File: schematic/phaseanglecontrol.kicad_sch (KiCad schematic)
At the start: 50 parts, among them J1 L_supply, J2 N_supply, J3 N_motor, J4 L_motor, K1 shutoff, U1 ATtiny26-16P, Y1 16 MHz

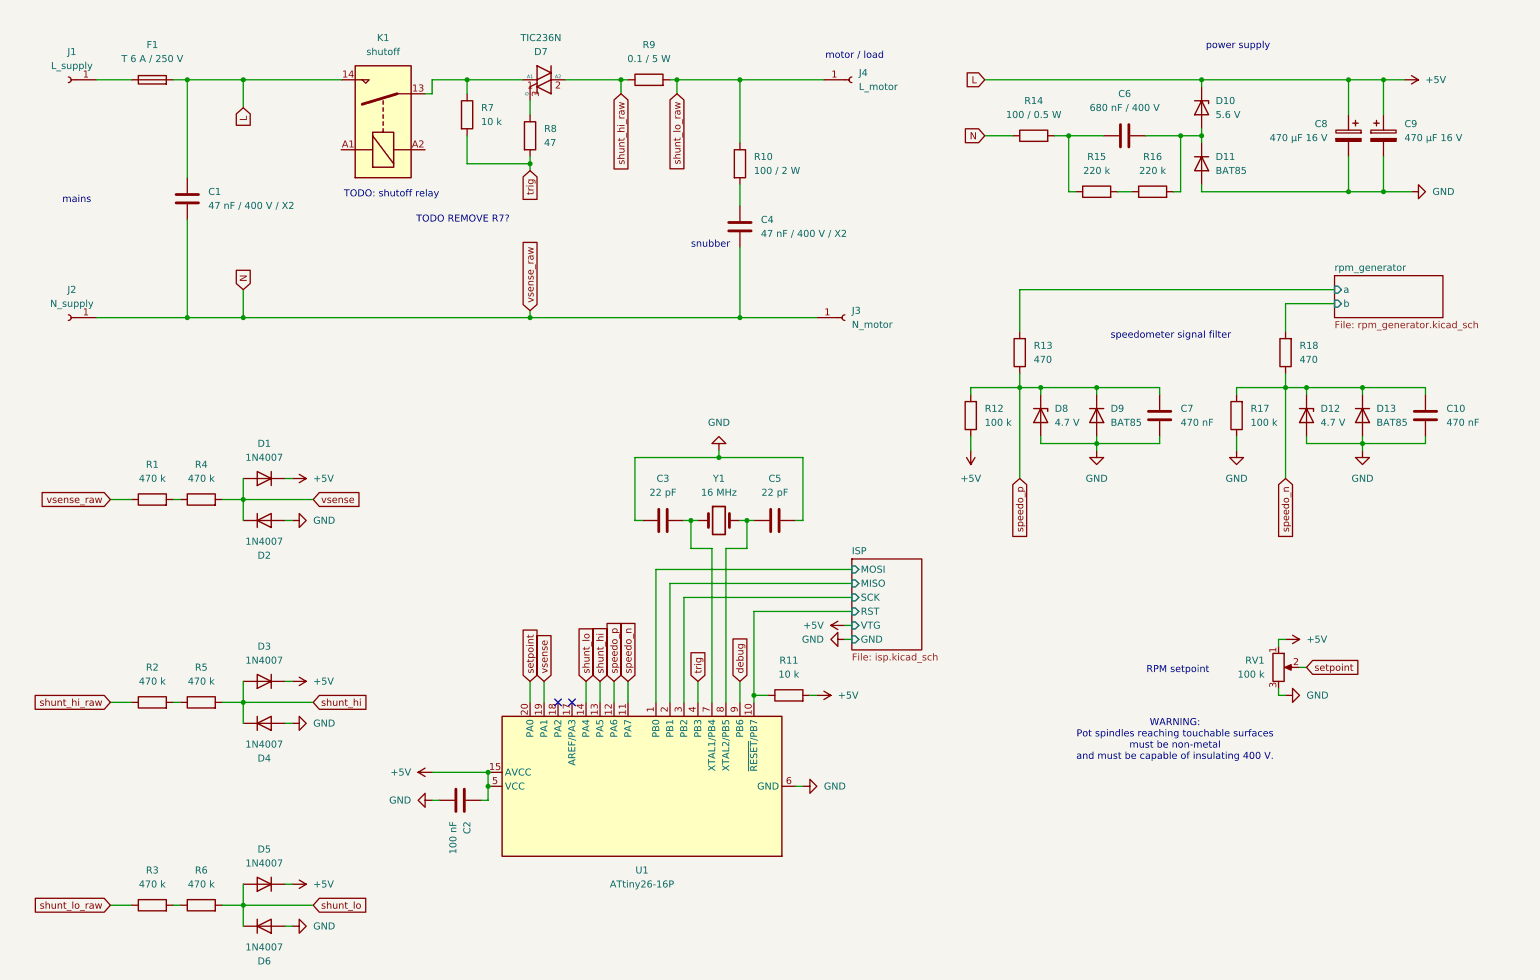
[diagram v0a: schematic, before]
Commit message: Update schematics
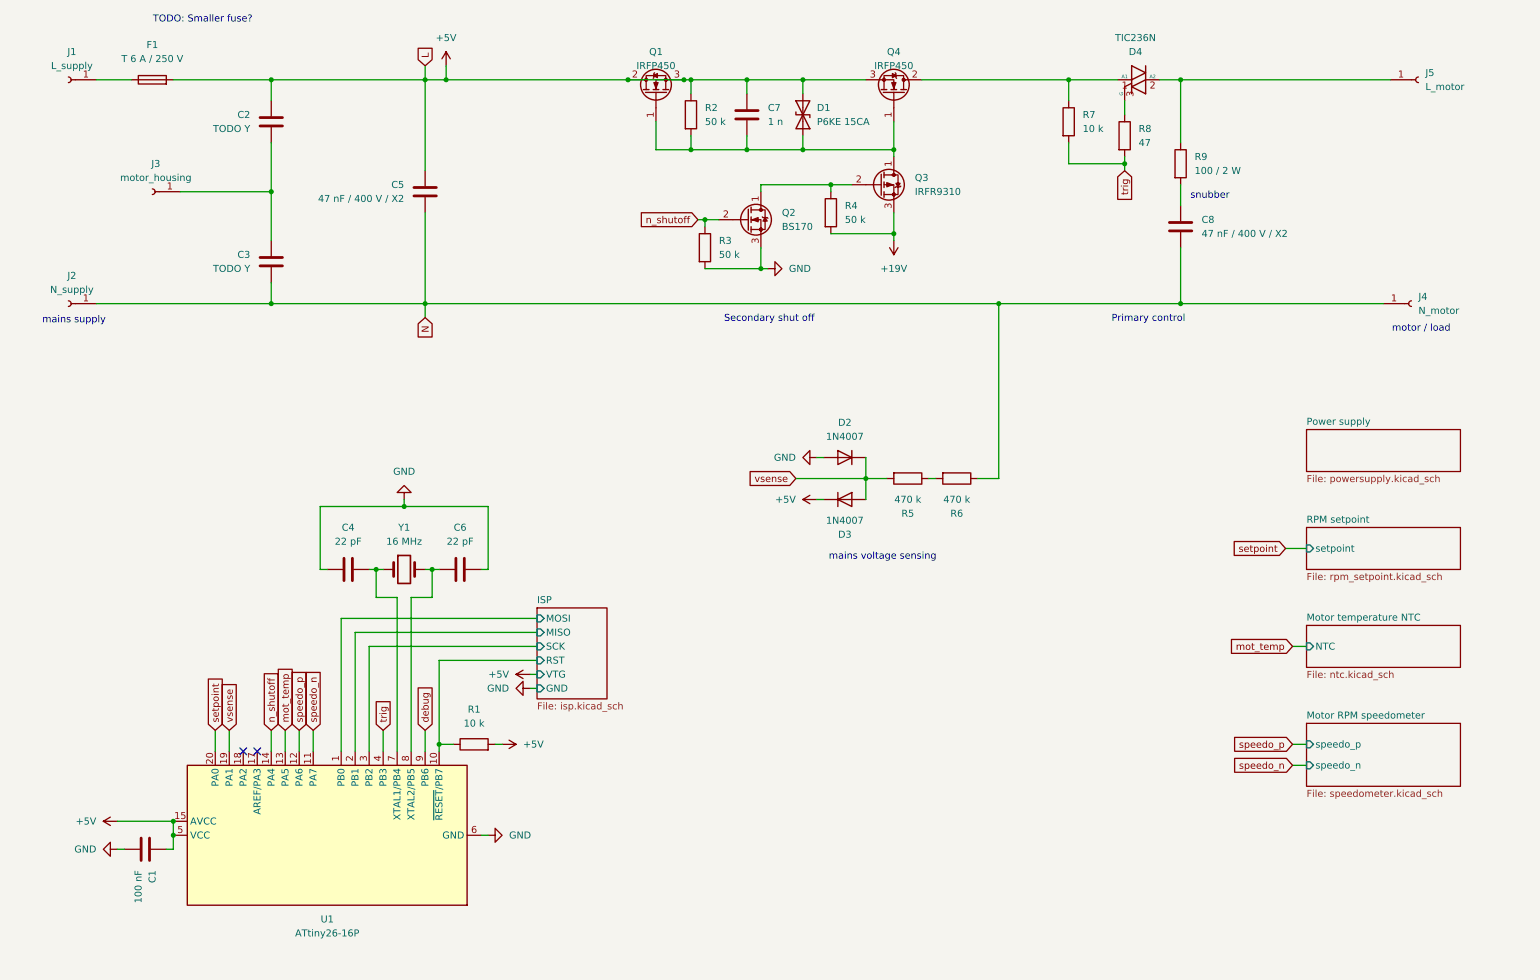
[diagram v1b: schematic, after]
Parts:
- removed C10: 470 nF, symbol Device:C
- removed C6: 680 nF / 400 V, symbol Device:C
- removed C8, C9: 470 µF 16 V, symbol Device:C_Polarized
- removed D10: 5.6 V, symbol Device:D_Zener
- removed D11, D13, D9: BAT85, symbol Device:D
- removed D12, D8: 4.7 V, symbol Device:D_Zener
- removed D3, D4, D5, D6: 1N4007, Diode_THT:D_DO-41_SOD81_P10.16mm_Horizontal, symbol Diode:1N4007
- removed K1: shutoff, symbol Relay:Relay_SPST-NO
- removed R12, R17: 100 k, symbol Device:R
- removed R13, R18: 470, symbol Device:R
- removed R14: 100 / 0.5 W, symbol Device:R
- removed R15, R16: 220 k, symbol Device:R
- removed R5, R6: 470 k, symbol Device:R
- removed R9: 0.1 / 5 W, symbol Device:R
- removed RV1: 100 k, symbol Device:R_Potentiometer
- added C2, C3: TODO Y, symbol Device:C
- added D1: P6KE 15CA, Diode_THT:D_DO-201AE_P15.24mm_Horizontal, symbol Diode:1N62xxCA
- added J3: motor_housing, symbol Connector:Conn_01x01_Socket
- added Q1, Q4: IRFP450, Package_TO_SOT_THT:TO-247-3_Vertical, symbol Transistor_FET:IRFP4468PbF
- added Q2: BS170, Package_TO_SOT_THT:TO-92_Inline, symbol Transistor_FET:BS170
- added Q3: IRFR9310, Package_TO_SOT_THT:TO-92_Inline, symbol Transistor_FET:BS250
- added R4: 50 k, symbol Device:R
- C7: value 470 nF -> 1 n
- R2, R3: value 470 k -> 50 k
- renumbered C2 to C1, C3 to C4, C1 to C5, C5 to C6, C4 to C8, D1 to D3, D7 to D4, J3 to J4, J4 to J5, R11 to R1, R4 to R5, R1 to R6, R10 to R9
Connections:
- net +5V: now also C7.1, R2.1, C2.2, D1.2 (A2), Q1.2 (D), Q1.3 (S), Q4.3 (S)
- net GND: now also R3.2, Q2.3 (S); no longer C7.2
- net N: now also C3.1
- net speedo_p: no longer C7.1
- net at D4.1 (A1), R7.1: now also Q4.2 (D)
- net at R2.2: now also C7.2, D1.1 (A1), Q1.1 (G), Q3.1 (D), Q4.1 (G)
- net shunt_hi renamed mot_temp
- net shunt_hi_raw: no longer names the net of D4.2 (A2)
- net shunt_hi_raw: now also J5.1 (Pin_1), R9.1; no longer R2.1
- net shunt_lo renamed n_shutoff
- net n_shutoff: now also R3.1, Q2.2 (G)
- removed net shunt_lo_raw: J5.1 (Pin_1), R3.1, R9.1
- new net: Q2.1 (D), Q3.2 (G), R4.1
- new net: C2.1, C3.2, J3.1 (Pin_1)
- new net +19V: Q3.3 (S), R4.2
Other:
- removed sheet rpm_generator
- added sheet Motor RPM speedometer (speedometer.kicad_sch)
- added sheet Motor temperature NTC (ntc.kicad_sch)
- added sheet Power supply (powersupply.kicad_sch)
- added sheet RPM setpoint (rpm_setpoint.kicad_sch)
- note added: "Primary control"
- note added: "Secondary shut off"
- note added: "TODO: Smaller fuse?"
- note added: "mains supply"
- note added: "mains voltage sensing"
- note removed: "RPM setpoint"
- note removed: "TODO REMOVE R7?"
- note removed: "TODO: shutoff relay"
- note removed: "WARNING: Pot spindles reaching touchable surfaces must be non-metal and must be capable of insulating 400 V."
- note removed: "mains"
- note removed: "power supply"
- note removed: "speedometer signal filter"
- moved on the sheet: C1, C4, C5, C6, C8, D2, D3, D4, J2, J4, J5, R1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

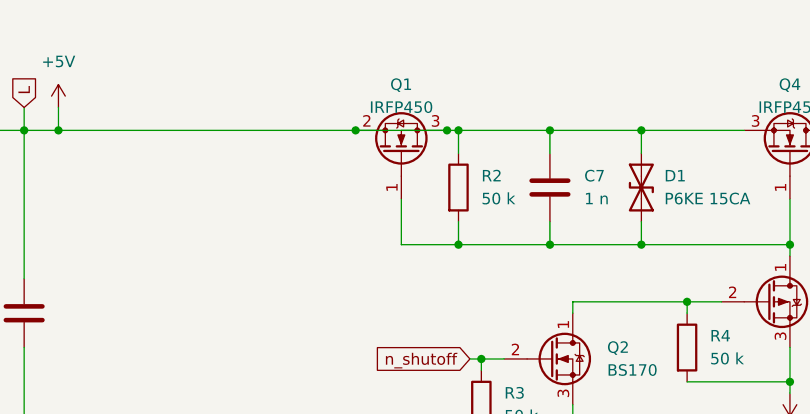
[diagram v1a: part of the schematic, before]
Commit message: Update schematic
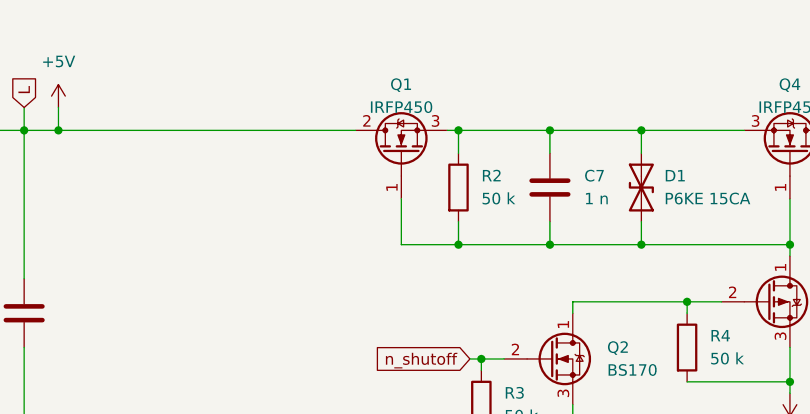
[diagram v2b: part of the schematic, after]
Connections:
- net +5V: no longer C7.1, D1.2 (A2), Q1.3 (S), Q4.3 (S), R2.1
- new net: C7.1, D1.2 (A2), Q1.3 (S), Q4.3 (S), R2.1
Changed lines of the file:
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@@
 	)
 	(junction
-		(at 135.89 27.94)
+		(at 137.16 27.94)
 		(diameter 0)
 		(color 0 0 0 0)
@@
 	)
 	(junction
-		(at 137.16 27.94)
-		(diameter 0)
-		(color 0 0 0 0)
-	)
-	(junction
 		(at 173.99 40.64)
 		(diameter 0)
@@
 	)
 	(junction
-		(at 125.73 27.94)
+		(at 92.71 27.94)
 		(diameter 0)
 		(color 0 0 0 0)
@@
 	(junction
 		(at 226.06 27.94)
-		(diameter 0)
-		(color 0 0 0 0)
-	)
-	(junction
-		(at 92.71 27.94)
 		(diameter 0)
 		(color 0 0 0 0)
@@
 	(wire
 		(pts
+			(xy 162.56 55.88) (xy 173.99 55.88)
+		)
+		(stroke
+			(width 0)
+			(type default)
+		)
+	)
+	(wire
+		(pts
+			(xy 222.25 27.94) (xy 226.06 27.94)
+		)
+		(stroke
+			(width 0)
+			(type default)
+		)
+	)
+	(wire
+		(pts
+			(xy 43.18 167.64) (xy 41.91 167.64)
+		)
+		(stroke
+			(width 0)
+			(type default)
+		)
+	)
+	(wire
+		(pts
+			(xy 149.86 62.23) (xy 151.13 62.23)
+		)
+		(stroke
+			(width 0)
+			(type default)
+		)
+	)
+	(wire
+		(pts
+			(xy 193.04 100.33) (xy 189.23 100.33)
+		)
+		(stroke
+			(width 0)
+			(type default)
+		)
+	)
+	(wire
+		(pts
+			(xy 130.81 40.64) (xy 137.16 40.64)
+		)
+		(stroke
+			(width 0)
+			(type default)
+		)
+	)
+	(wire
+		(pts
+			(xy 33.02 167.64) (xy 34.29 167.64)
+		)
+		(stroke
+			(width 0)
+			(type default)
+		)
+	)
+	(wire
+		(pts
+			(xy 173.99 40.64) (xy 173.99 35.56)
+		)
+		(stroke
+			(width 0)
+			(type default)
+		)
+	)
+	(wire
+		(pts
+			(xy 168.91 104.14) (xy 168.91 100.33)
+		)
+		(stroke
+			(width 0)
+			(type default)
+		)
+	)
+	(wire
+		(pts
+			(xy 83.82 121.92) (xy 83.82 149.86)
+		)
+		(stroke
+			(width 0)
+			(type default)
+		)
+	)
+	(wire
+		(pts
+			(xy 60.96 27.94) (xy 60.96 31.75)
+		)
+		(stroke
+			(width 0)
+			(type default)
+		)
+	)
+	(wire
+		(pts
+			(xy 157.48 27.94) (xy 168.91 27.94)
+		)
+		(stroke
+			(width 0)
+			(type default)
+		)
+	)
+	(wire
+		(pts
+			(xy 172.72 100.33) (xy 168.91 100.33)
+		)
+		(stroke
+			(width 0)
+			(type default)
+		)
+	)
+	(wire
+		(pts
+			(xy 90.17 121.92) (xy 86.36 121.92)
+		)
+		(stroke
+			(width 0)
+			(type default)
+		)
+	)
+	(wire
+		(pts
+			(xy 168.91 100.33) (xy 156.21 100.33)
+		)
+		(stroke
+			(width 0)
+			(type default)
+		)
+	)
+	(wire
+		(pts
+			(xy 226.06 58.42) (xy 226.06 68.58)
+		)
+		(stroke
+			(width 0)
+			(type default)
+		)
+	)
+	(wire
+		(pts
+			(xy 68.58 146.05) (xy 68.58 149.86)
+		)
+		(stroke
+			(width 0)
+			(type default)
+		)
+	)
+	(wire
+		(pts
+			(xy 43.18 27.94) (xy 60.96 27.94)
+		)
+		(stroke
+			(width 0)
+			(type default)
+		)
+	)
+	(wire
+		(pts
+			(xy 43.18 162.56) (xy 43.18 165.1)
+		)
+		(stroke
+			(width 0)
+			(type default)
+		)
+	)
+	(wire
+		(pts
+			(xy 205.74 39.37) (xy 205.74 43.18)
+		)
+		(stroke
+			(width 0)
+			(type default)
+		)
+	)
+	(wire
+		(pts
+			(xy 60.96 27.94) (xy 88.9 27.94)
+		)
+		(stroke
+			(width 0)
+			(type default)
+		)
+	)
+	(wire
+		(pts
 			(xy 92.71 27.94) (xy 125.73 27.94)
 		)
@@
 	(wire
 		(pts
-			(xy 162.56 55.88) (xy 173.99 55.88)
-		)
-		(stroke
-			(width 0)
-			(type default)
-		)
-	)
-	(wire
-		(pts
-			(xy 222.25 27.94) (xy 226.06 27.94)
-		)
-		(stroke
-			(width 0)
-			(type default)
-		)
-	)
-	(wire
-		(pts
-			(xy 137.16 27.94) (xy 135.89 27.94)
-		)
-		(stroke
-			(width 0)
-			(type default)
-		)
-	)
-	(wire
-		(pts
-			(xy 43.18 167.64) (xy 41.91 167.64)
-		)
-		(stroke
-			(width 0)
-			(type default)
-		)
-	)
-	(wire
-		(pts
-			(xy 149.86 62.23) (xy 151.13 62.23)
-		)
-		(stroke
-			(width 0)
-			(type default)
-		)
-	)
-	(wire
-		(pts
-			(xy 193.04 100.33) (xy 189.23 100.33)
-		)
-		(stroke
-			(width 0)
-			(type default)
-		)
-	)
-	(wire
-		(pts
-			(xy 130.81 40.64) (xy 137.16 40.64)
-		)
-		(stroke
-			(width 0)
-			(type default)
-		)
-	)
-	(wire
-		(pts
-			(xy 33.02 167.64) (xy 34.29 167.64)
-		)
-		(stroke
-			(width 0)
-			(type default)
-		)
-	)
-	(wire
-		(pts
-			(xy 173.99 40.64) (xy 173.99 35.56)
-		)
-		(stroke
-			(width 0)
-			(type default)
-		)
-	)
-	(wire
-		(pts
-			(xy 168.91 104.14) (xy 168.91 100.33)
-		)
-		(stroke
-			(width 0)
-			(type default)
-		)
-	)
-	(wire
-		(pts
-			(xy 83.82 121.92) (xy 83.82 149.86)
-		)
-		(stroke
-			(width 0)
-			(type default)
-		)
-	)
-	(wire
-		(pts
-			(xy 60.96 27.94) (xy 60.96 31.75)
-		)
-		(stroke
-			(width 0)
-			(type default)
-		)
-	)
-	(wire
-		(pts
-			(xy 157.48 27.94) (xy 168.91 27.94)
-		)
-		(stroke
-			(width 0)
-			(type default)
-		)
-	)
-	(wire
-		(pts
-			(xy 172.72 100.33) (xy 168.91 100.33)
-		)
-		(stroke
-			(width 0)
-			(type default)
-		)
-	)
-	(wire
-		(pts
-			(xy 90.17 121.92) (xy 86.36 121.92)
-		)
-		(stroke
-			(width 0)
-			(type default)
-		)
-	)
-	(wire
-		(pts
-			(xy 168.91 100.33) (xy 156.21 100.33)
-		)
-		(stroke
-			(width 0)
-			(type default)
-		)
-	)
-	(wire
-		(pts
-			(xy 226.06 58.42) (xy 226.06 68.58)
-		)
-		(stroke
-			(width 0)
-			(type default)
-		)
-	)
-	(wire
-		(pts
-			(xy 68.58 146.05) (xy 68.58 149.86)
-		)
-		(stroke
-			(width 0)
-			(type default)
-		)
-	)
-	(wire
-		(pts
-			(xy 43.18 27.94) (xy 60.96 27.94)
-		)
-		(stroke
-			(width 0)
-			(type default)
-		)
-	)
-	(wire
-		(pts
-			(xy 43.18 162.56) (xy 43.18 165.1)
-		)
-		(stroke
-			(width 0)
-			(type default)
-		)
-	)
-	(wire
-		(pts
-			(xy 205.74 39.37) (xy 205.74 43.18)
-		)
-		(stroke
-			(width 0)
-			(type default)
-		)
-	)
-	(wire
-		(pts
-			(xy 135.89 27.94) (xy 125.73 27.94)
-		)
-		(stroke
-			(width 0)
-			(type default)
-		)
-	)
-	(wire
-		(pts
-			(xy 60.96 27.94) (xy 88.9 27.94)
-		)
-		(stroke
-			(width 0)
-			(type default)
-		)
-	)
-	(wire
-		(pts
 			(xy 80.01 116.84) (xy 80.01 121.92)
 		)
@@
 		)
 		(stroke
+			(width 0)
+			(type default)
+		)
+	)
+	(wire
+		(pts
+			(xy 135.89 27.94) (xy 137.16 27.94)
+		)
+		(stroke
